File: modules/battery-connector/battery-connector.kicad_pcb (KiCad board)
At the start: 2 copper layers, 15 x 12.7 mm, 2 parts, among them J1 691210910002

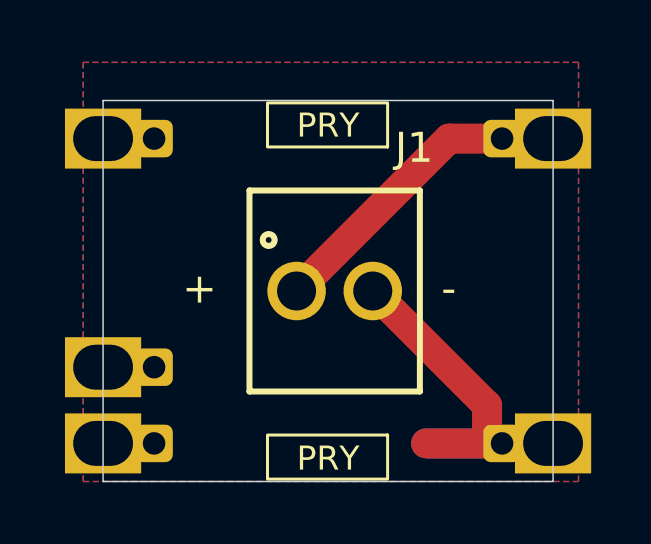
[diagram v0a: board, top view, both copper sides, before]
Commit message: Update one board - checking workflow
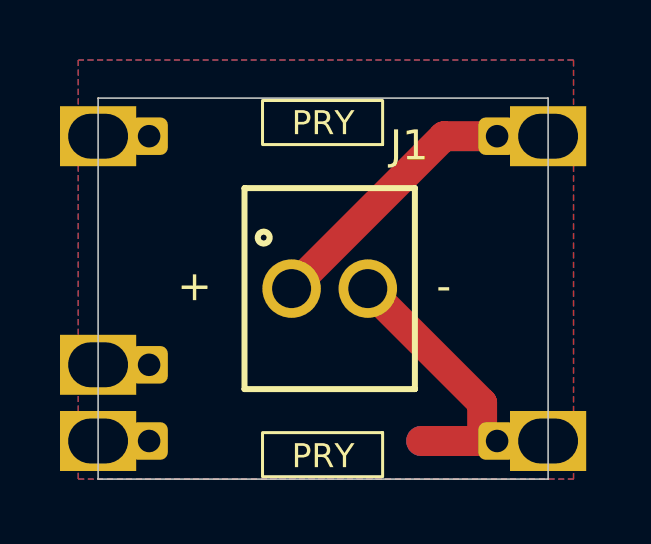
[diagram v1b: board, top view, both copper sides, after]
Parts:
- moved J1 0.18 mm to (67.9, 60.9)
- moved M1 0.18 mm to (67.7, 60.9)
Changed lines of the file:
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@@
 	(footprint "MegaCastle:691210910002"
 		(layer "F.Cu")
-		(at 68.072 60.96)
+		(at 67.906 60.88)
 		(descr "<b>WR-TBL Serie 2109 - 2.54 mm Horiz. Entry<br></b>Max Height =8.5mm , Pitch 2.54mm , 2 Pins")
 		(property "Reference" "J1"
@@
 	(footprint "MegaCastle:MegaCastle2x5-Module-I15.0x7.9-M8CC-SPAREPAD"
 		(layer "B.Cu")
-		(at 67.852 60.96 180)
+		(at 67.686 60.88 180)
 		(property "Reference" "M1"
 			(at -2.948 -5.65 0)
@@
 			(polygon
 				(pts
-					(xy 69.836241 56.158592) (xy 69.836241 54.69) (xy 65.832484 54.69) (xy 65.832484 56.158592)
+					(xy 69.670241 56.078592) (xy 69.670241 54.61) (xy 65.666484 54.61) (xy 65.666484 56.078592)
 				)
 			)
@@
 			(polygon
 				(pts
-					(xy 69.836241 65.761408) (xy 69.836241 67.23) (xy 65.832484 67.23) (xy 65.832484 65.761408)
+					(xy 69.670241 65.681408) (xy 69.670241 67.15) (xy 65.666484 67.15) (xy 65.666484 65.681408)
 				)
 			)
@@
 			(polygon
 				(pts
-					(xy 75.352 54.61) (xy 75.352 57.01) (xy 60.352 57.01) (xy 60.352 54.61)
+					(xy 75.186 54.53) (xy 75.186 56.93) (xy 60.186 56.93) (xy 60.186 54.53)
 				)
 			)
@@
 			(polygon
 				(pts
-					(xy 75.352 67.31) (xy 75.352 64.91) (xy 60.352 64.91) (xy 60.352 67.31)
+					(xy 75.186 67.23) (xy 75.186 64.83) (xy 60.186 64.83) (xy 60.186 67.23)
 				)
 			)
@@
 	)
 	(gr_text "-"
-		(at 71.628 61.468 0)
+		(at 71.462 61.388 0)
 		(layer "F.SilkS")
 		(effects
@@
 	)
 	(gr_text "+"
-		(at 62.992 61.468 0)
+		(at 62.826 61.388 0)
 		(layer "F.SilkS")
 		(effects
@@
 	)
 	(gr_text "R20250405"
-		(at 65.1256 57.7342 90)
+		(at 64.9596 57.6542 90)
 		(layer "B.SilkS")
 		(effects
@@
 	)
 	(segment
-		(start 73.152 55.88)
-		(end 71.882 55.88)
+		(start 72.986 55.8)
+		(end 71.716 55.8)
 		(width 1)
 		(layer "F.Cu")
@@
 	)
 	(segment
-		(start 71.882 55.88)
-		(end 66.802 60.96)
+		(start 71.716 55.8)
+		(end 66.636 60.88)
 		(width 1)
 		(layer "F.Cu")
@@
 	)
 	(segment
-		(start 73.152 66.04)
-		(end 73.152 64.77)
+		(start 72.986 65.96)
+		(end 72.986 64.69)
 		(width 1)
 		(layer "F.Cu")
@@
 	)
 	(segment
-		(start 73.152 64.77)
-		(end 69.342 60.96)
+		(start 72.986 64.69)
+		(end 69.176 60.88)
 		(width 1)
 		(layer "F.Cu")
@@
 	)
 	(segment
-		(start 73.152 66.04)
-		(end 71.12 66.04)
+		(start 72.986 65.96)
+		(end 70.954 65.96)
 		(width 1)
 		(layer "F.Cu")
@@
 	)
 	(segment
-		(start 73.152 66.04)
-		(end 71.12 66.04)
+		(start 72.986 65.96)
+		(end 70.954 65.96)
 		(width 1)
 		(layer "B.Cu")
@@
 		(polygon
 			(pts
-				(xy 59.69 53.34) (xy 59.69 67.31) (xy 76.2 67.31) (xy 76.2 53.34)
-			)
-		)
+				(xy 59.524 53.26) (xy 59.524 67.23) (xy 76.034 67.23) (xy 76.034 53.26)
+			)
+		)
